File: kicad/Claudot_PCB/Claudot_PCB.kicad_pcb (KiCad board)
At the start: 2 copper layers, 104.8 x 57.2 mm, 31 parts, among them J1 Conn_01x08

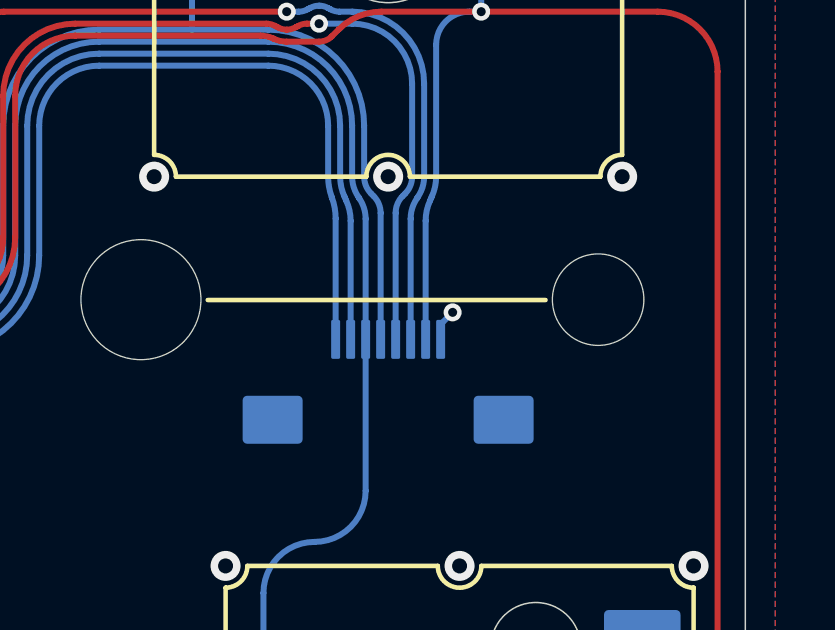
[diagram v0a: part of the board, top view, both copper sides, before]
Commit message: feat: finalize Claudot_PCB and Claudot_MCU
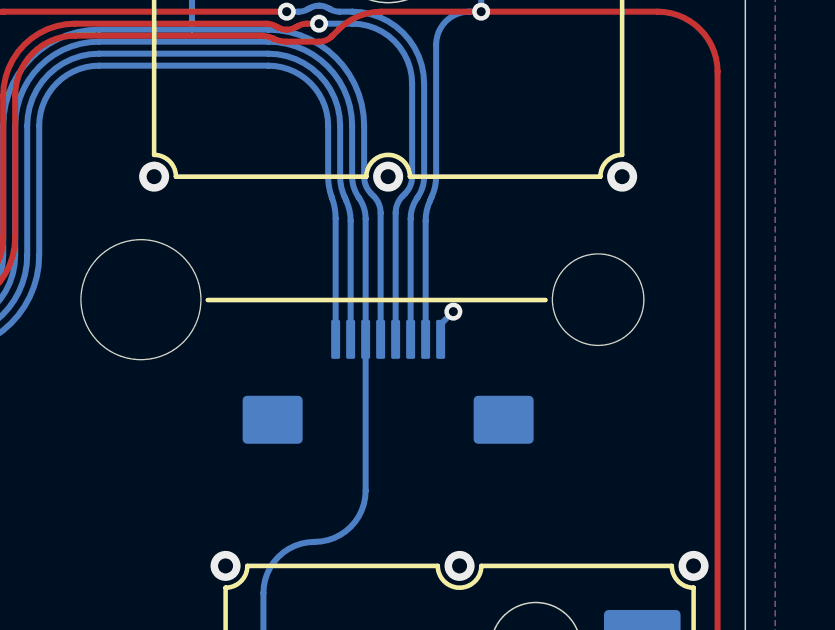
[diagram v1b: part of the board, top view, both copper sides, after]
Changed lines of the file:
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@@
 	(gr_line
 		(start 142.24375 79.3985)
-		(end 142.64375 78.9985)
+		(end 142.668014 78.974236)
 		(stroke
 			(width 0.2)
@@
 	)
 	(via
-		(at 142.64375 78.9985)
+		(at 142.668014 78.974236)
 		(size 0.6)
 		(drill 0.3)
